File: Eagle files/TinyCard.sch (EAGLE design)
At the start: 35 parts, among them CN1 USBA_FEMALE, IC1 MAX619CSA, Q1 MOSFET-PCHANNELSMD, U5 SD_CARD_SOCKET4UCON

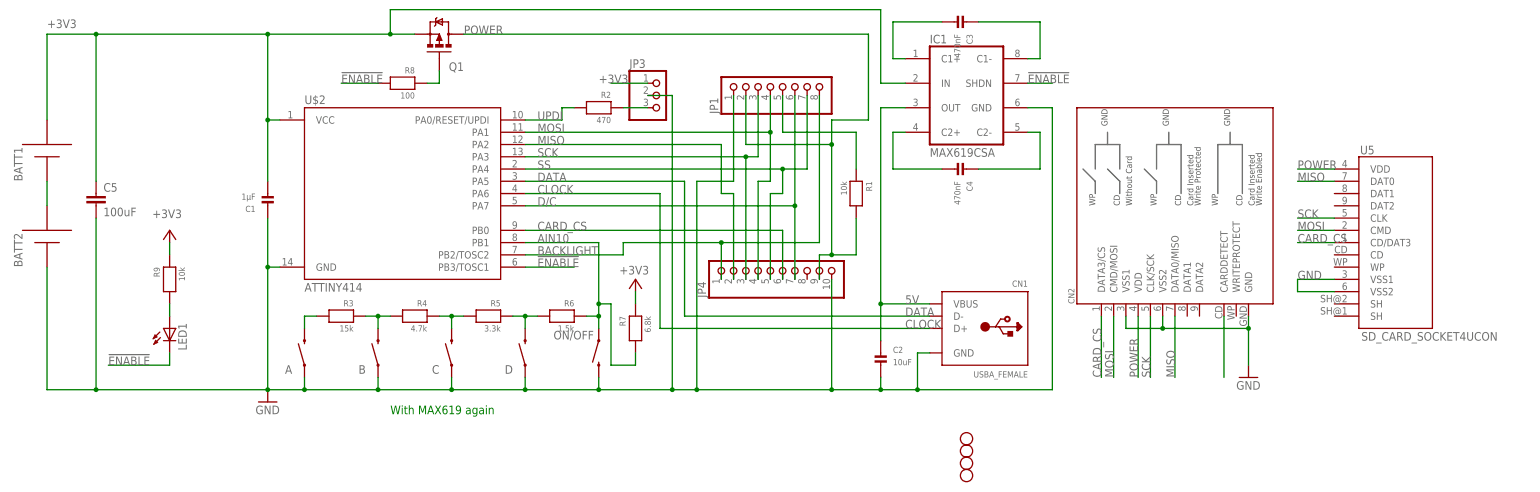
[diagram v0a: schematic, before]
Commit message: Version 2 - 27th March 2025
Decoupling capacitors
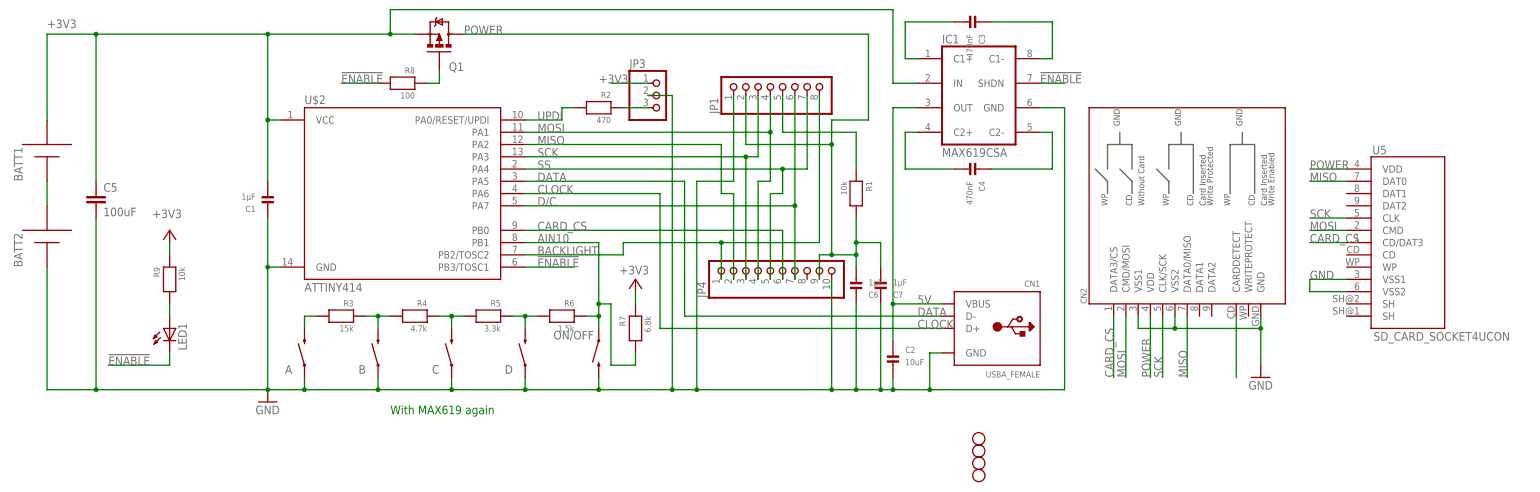
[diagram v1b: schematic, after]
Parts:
- added C6, C7: 1µF, microbuilder:CAP_CERAMIC_0805MP
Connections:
- net GND: now also C6.P$1, C7.P$1
- net POWER: now also C6.P$2, C7.P$2
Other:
- moved on the sheet: C2, C3, C4, CN1, CN2, IC1, U5
